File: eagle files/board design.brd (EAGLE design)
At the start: 168.9 x 116.5 mm, 35 parts

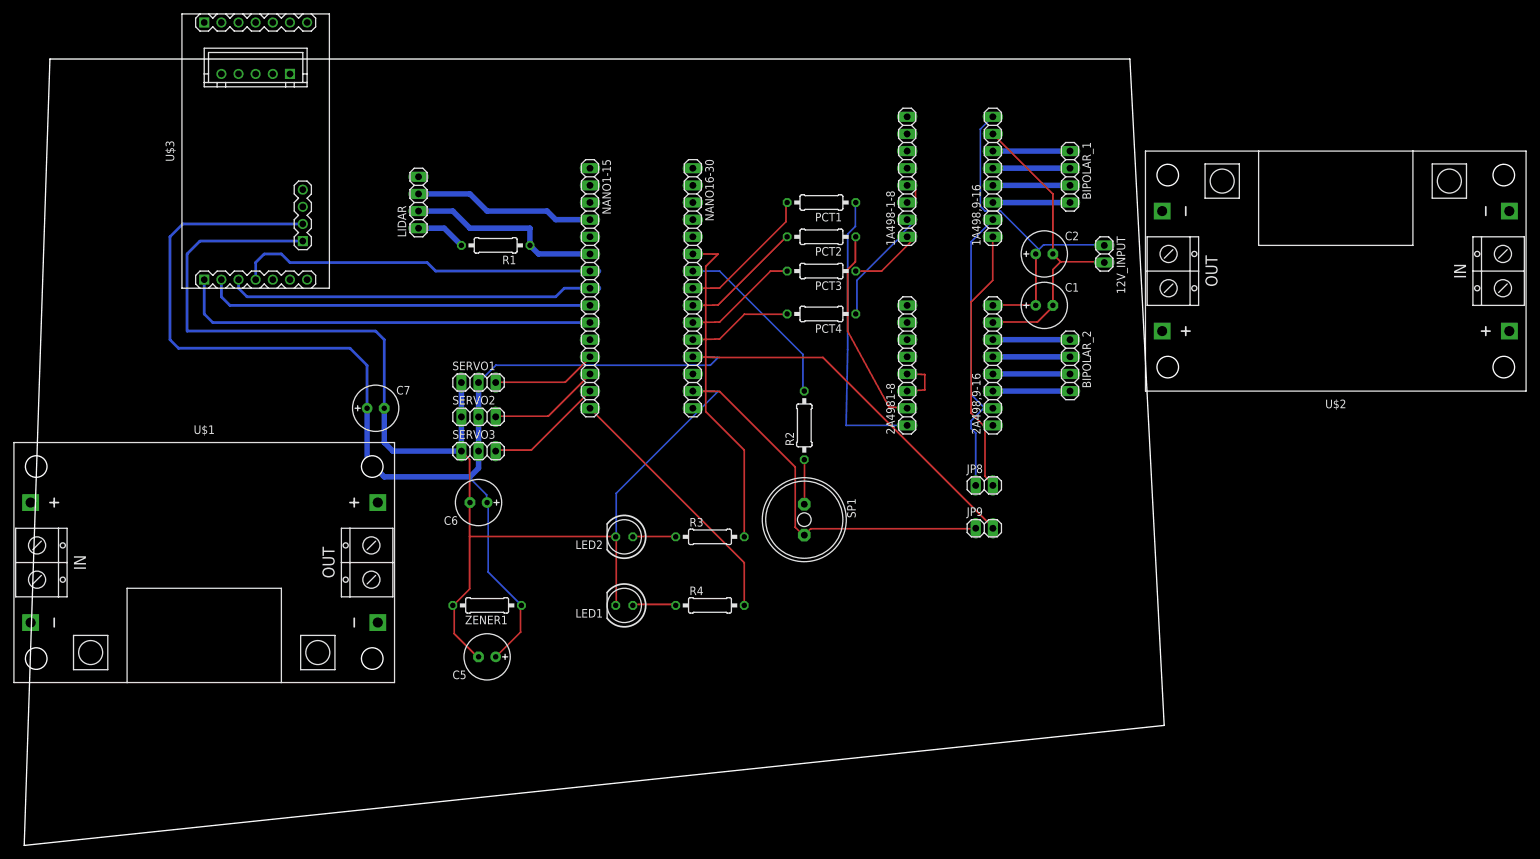
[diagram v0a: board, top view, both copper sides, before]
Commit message: 10/2/19
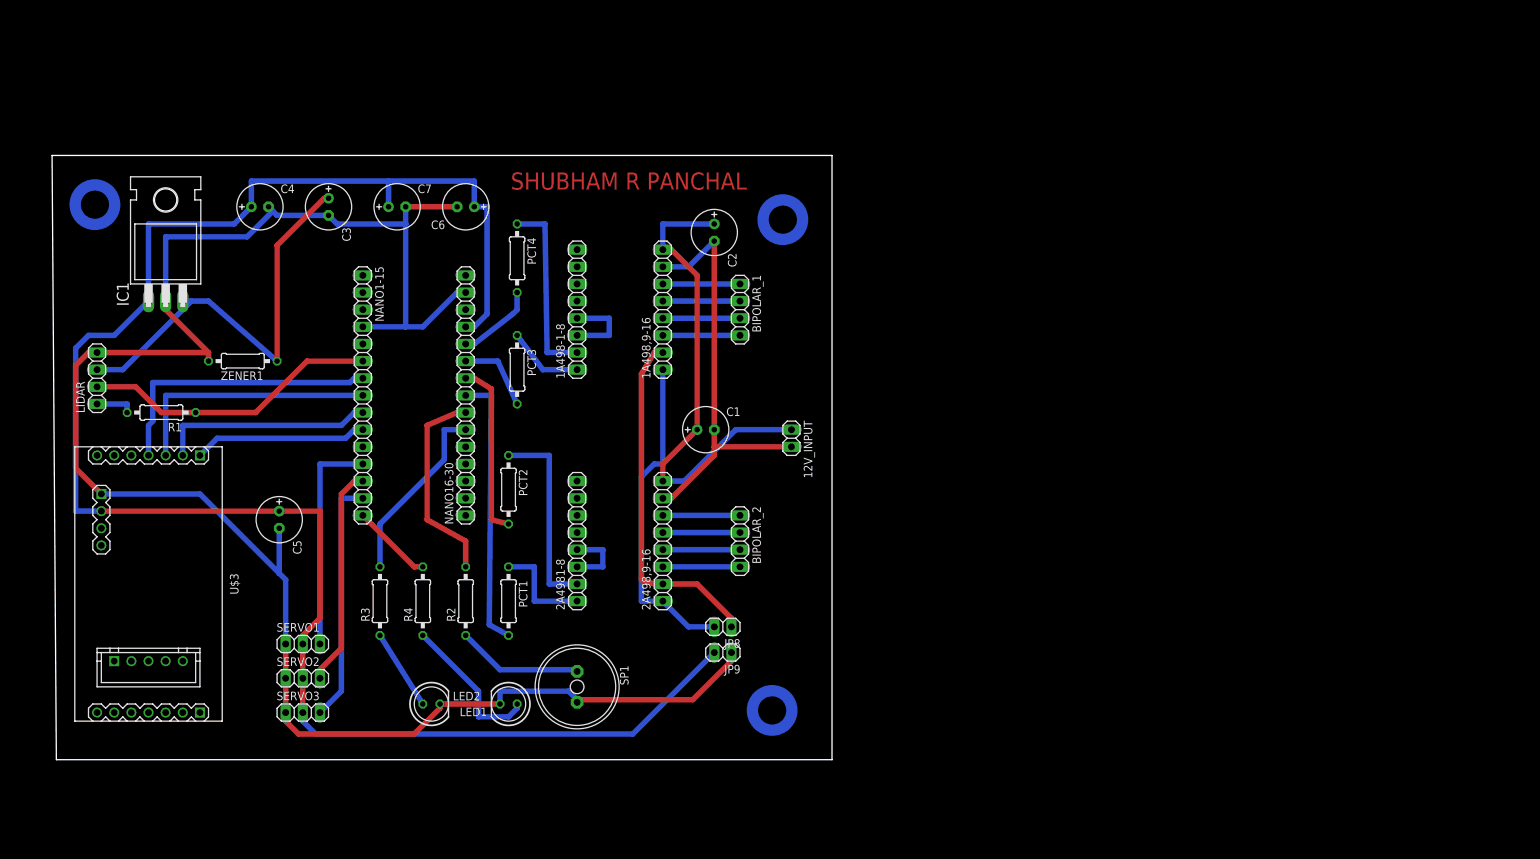
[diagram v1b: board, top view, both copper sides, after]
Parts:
- removed U$1, U$2: DC-DC-LM2596-DISP, uln2003:DC-DC-LM2596-DISP
- added C3, C4: (no value), rcl:E2,5-7
- added IC1: 7805T, linear:TO220H
- moved PCT1 75.1 mm to (67.9, 19.7), turned to 270 degrees
- moved U$3 66.1 mm to (14.6, 22.2), turned to 270 degrees
- moved PCT2 59.6 mm to (67.9, 36.2), turned to 270 degrees
- moved R2 56.5 mm to (61.6, 19.7)
- moved 2A4981-8 55.4 mm to (78.1, 28.6)
- moved BIPOLAR_2 55.4 mm to (102.2, 28.6)
- moved 2A498,9-16 55.4 mm to (90.8, 28.6)
- moved R1 55.4 mm to (16.5, 47.6)
- moved LIDAR 54.3 mm to (6.99, 52.7)
- moved 12V_INPUT 53.8 mm to (109.9, 43.8)
- moved C1 53.4 mm to (97.2, 45.1)
- moved 1A498-1-8 52.7 mm to (78.1, 62.9)
- moved BIPOLAR_1 52.7 mm to (102.2, 62.9)
- moved 1A498,9-16 52.7 mm to (90.8, 62.9)
- moved ZENER1 51.2 mm to (28.6, 55.2)
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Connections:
- new net N$37: C3.+, IC1.3, LIDAR.3, ZENER1.1
- net 5V: now also C4.+, IC1.1; no longer LIDAR.4, ZENER1.1
- net GND: now also C3.-, C4.-, IC1.2, LIDAR.4; no longer LIDAR.3
- net N$22: no longer U$2.OUT-
- net N$25: no longer U$2.OUT+
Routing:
- net N$37: track 0.00 -> 63.1 mm
- net N$4: track 62.8 -> 25.7 mm
- net 5V: track 238.5 -> 266.8 mm
- net N$32: track 42.6 -> 15.2 mm
- net N$18: track 38.7 -> 12.0 mm
- net N$3: track 57.7 -> 31.9 mm
- net N$33: track 48.7 -> 27.4 mm
- net N$25: track 52.6 -> 72.9 mm
- net N$8: track 20.8 -> 41.1 mm
- net N$28: track 17.7 -> 36.2 mm
- net N$2: track 55.7 -> 38.1 mm
- net N$26: track 15.6 -> 33.0 mm
- net N$27: track 16.7 -> 32.6 mm
- net N$17: track 6.53 -> 22.4 mm
- net N$20: track 29.5 -> 44.1 mm
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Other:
- board size 168.9 x 116.5 mm -> 115.6 x 89.5 mm
- board text added: "SHUBHAM R PANCHAL"
